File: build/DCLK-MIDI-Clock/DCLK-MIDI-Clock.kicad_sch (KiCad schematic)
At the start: 24 parts, among them J1 MIDI OUT, J2 Jack-DC, J3 MIDI OUT, SW1 CH1, SW2 CH2, SW3 SETTINGS, SW4 RotaryEncoder_Switch_MP

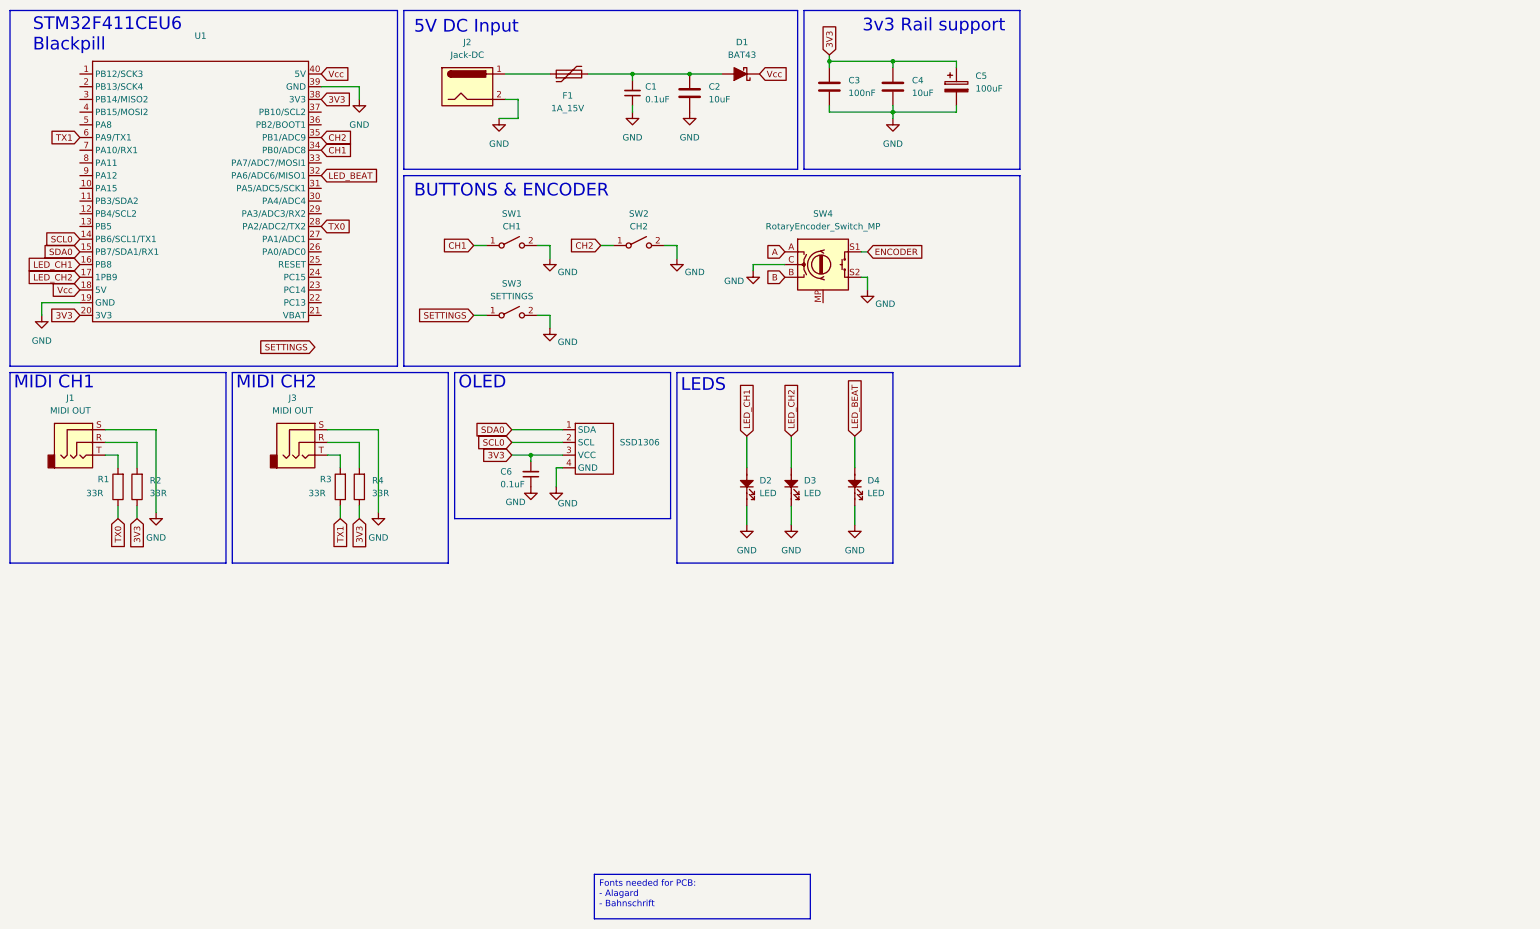
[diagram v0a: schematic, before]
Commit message: pcb rev2
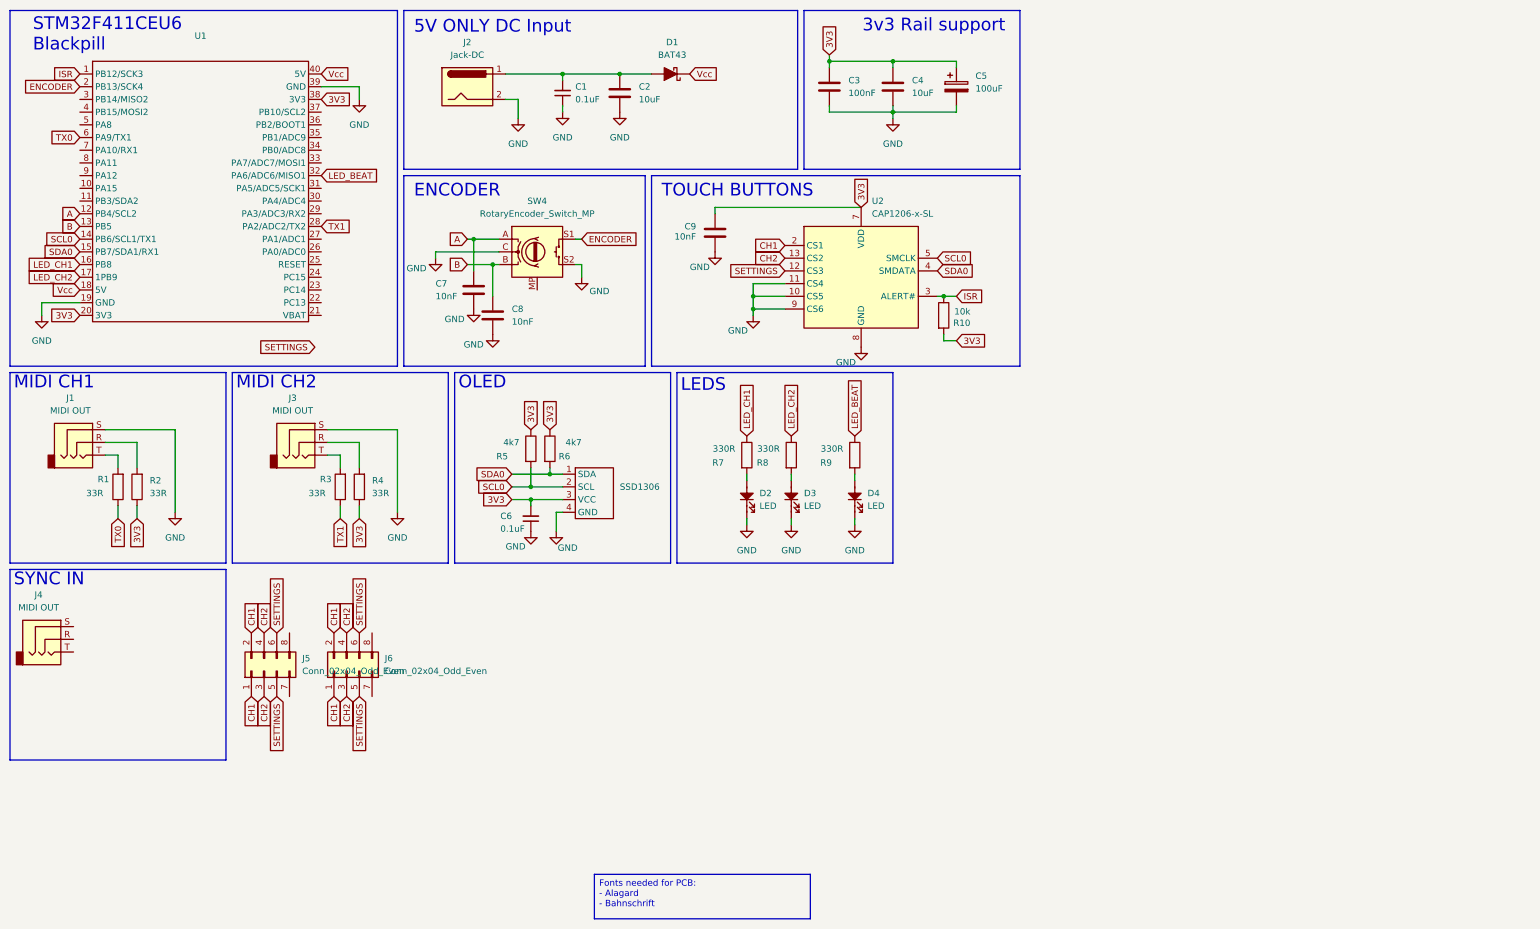
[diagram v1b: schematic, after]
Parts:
- removed F1: 1A_15V, Fuse:Fuse_1812_4532Metric, symbol PCM_4ms_Regulator:Polyfuse_3A_15V
- removed SW1: CH1, Button_Switch_Keyboard:SW_Cherry_MX_1.00u_PCB, symbol Switch:SW_SPST
- removed SW2: CH2, Button_Switch_Keyboard:SW_Cherry_MX_1.00u_PCB, symbol Switch:SW_SPST
- removed SW3: SETTINGS, Button_Switch_Keyboard:SW_Cherry_MX_1.00u_PCB, symbol Switch:SW_SPST
- added C7, C8, C9: 10nF, Capacitor_SMD:C_1206_3216Metric_Pad1.33x1.80mm_HandSolder, symbol Device:C
- added J4: MIDI OUT, audioConnectors_Edit:Jack_3.5mm_CUI_SJ1-3525N_Horizontal_edit, symbol Connector_Audio:AudioJack3
- added J5: Conn_02x04_Odd_Even, Connector_PinSocket_2.54mm:PinSocket_2x04_P2.54mm_Vertical, symbol Connector_Generic:Conn_02x04_Odd_Even
- added J6: Conn_02x04_Odd_Even, Connector_PinHeader_2.54mm:PinHeader_2x04_P2.54mm_Vertical_SMD, symbol Connector_Generic:Conn_02x04_Odd_Even
- added R10: 10k, PCM_4ms_Resistor:R_0603, symbol PCM_4ms_Resistor:10k_0402
- added R5, R6: 4k7, PCM_4ms_Resistor:R_0603, symbol PCM_4ms_Resistor:10k_0402
- added R7, R8, R9: 330R, PCM_4ms_Resistor:R_0603, symbol PCM_4ms_Resistor:10k_0402
- added U2: CAP1206-x-SL, Package_SO:SOIC-14_3.9x8.7mm_P1.27mm, symbol Sensor_Touch:CAP1206-x-SL
- SSD1306: footprint SSD1306_footprint:SSD1306_OLED_Module -> SSD1306:SSD1306-128x32
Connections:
- net 3V3: now also C9.2, R10.2, R5.1, R6.1, U2.7 (VDD)
- net A: now also U1.12 (PB4/SCL2), C7.1
- net B: now also U1.13 (PB5), C8.1
- net CH1: now also J5.1 (Pin_1), J5.2 (Pin_2), J6.1 (Pin_1), J6.2 (Pin_2), U2.2 (CS1); no longer U1.34 (PB0/ADC8)
- net CH2: now also J5.3 (Pin_3), J5.4 (Pin_4), J6.3 (Pin_3), J6.4 (Pin_4), U2.13 (CS2); no longer U1.35 (PB1/ADC9)
- net ENCODER: now also U1.2 (PB13/SCK4)
- net GND: now also C7.2, C8.2, C9.1, U2.10 (CS5), U2.11 (CS4), U2.8 (GND), U2.9 (CS6)
- net LED_BEAT: now also R9.1; no longer D4.2
- net LED_CH1: now also R7.1; no longer D2.2
- net LED_CH2: now also R8.1; no longer D3.2
- net SCL0: now also R5.2, U2.5 (SMCLK)
- net SDA0: now also R6.2, U2.4 (SMDATA)
- net SETTINGS: now also J5.5 (Pin_5), J5.6 (Pin_6), J6.5 (Pin_5), J6.6 (Pin_6), U2.12 (CS3)
- net TX0: now also U1.6 (PA9/TX1); no longer U1.28 (PA2/ADC2/TX2)
- net TX1: now also U1.28 (PA2/ADC2/TX2); no longer U1.6 (PA9/TX1)
- net ISR: now reaches U1.1 (PB12/SCK3)
- net ISR: now also R10.1, U2.3 (ALERT#)
- net at C1.2, C2.1, D1.2 (A): now also J2.1
- new net: D3.2, R8.2
- new net: D4.2, R9.2
- new net: D2.2, R7.2
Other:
- note added: "5V ONLY DC Input"
- note added: "ENCODER"
- note added: "SYNC IN"
- note added: "TOUCH BUTTONS"
- note removed: "5V DC Input"
- note removed: "BUTTONS & ENCODER"
- moved on the sheet: C1, C2, C6, D1, D2, D3, D4, SSD1306, SW4

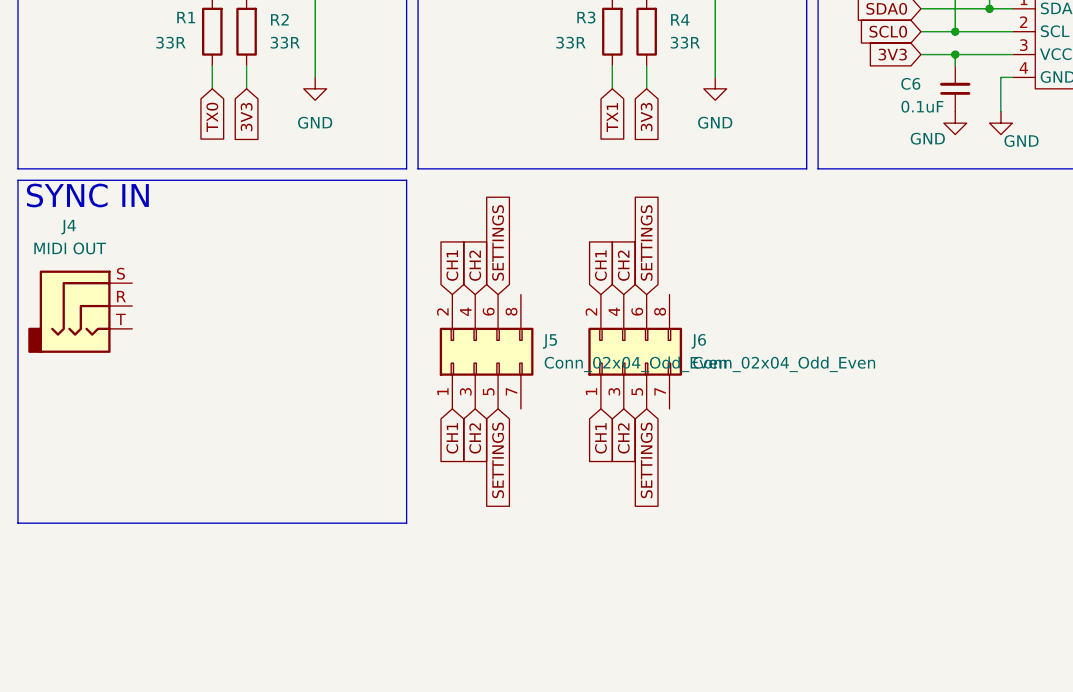
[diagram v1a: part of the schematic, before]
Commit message: pcb rev2
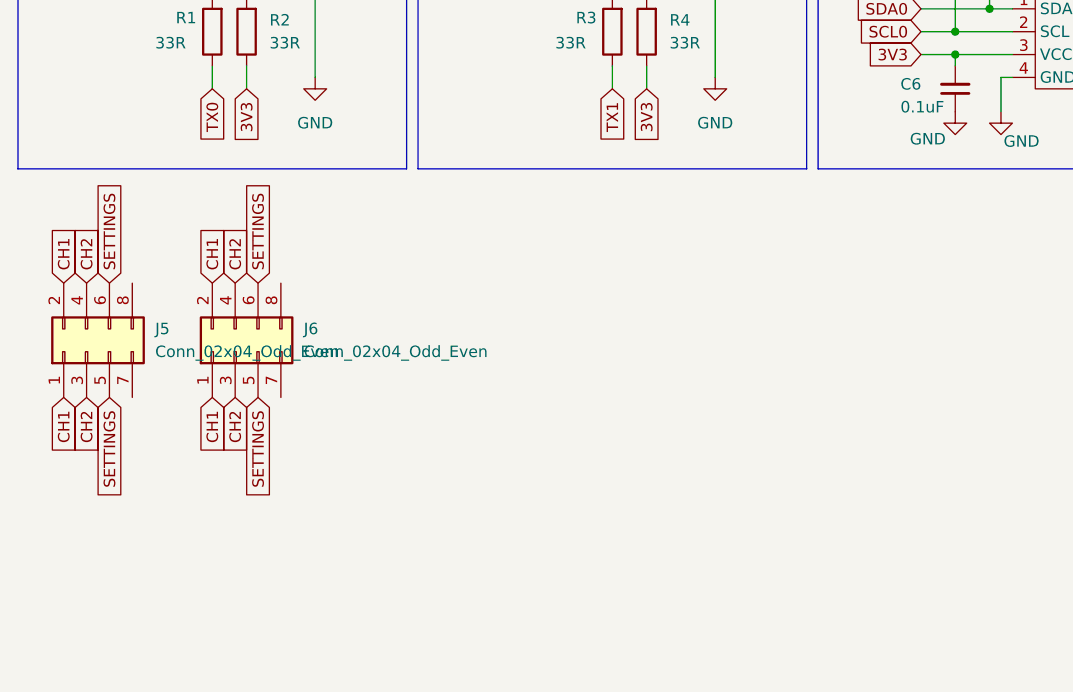
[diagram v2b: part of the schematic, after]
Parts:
- removed J4: MIDI OUT, audioConnectors_Edit:Jack_3.5mm_CUI_SJ1-3525N_Horizontal_edit, symbol Connector_Audio:AudioJack3
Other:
- note removed: "SYNC IN"
- moved on the sheet: J5, J6
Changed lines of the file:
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@@
 	)
 	(rectangle
-		(start 13.97 125.73)
-		(end 57.15 163.83)
-		(stroke
-			(width 0)
-			(type default)
-		)
-		(fill
-			(type none)
-		)
-	)
-	(rectangle
 		(start 102.87 86.36)
 		(end 146.05 124.46)
@@
 		)
 	)
-	(text "SYNC IN"
-		(exclude_from_sim no)
-		(at 14.732 127.762 0)
-		(effects
-			(font
-				(face "Alagard")
-				(size 2.54 2.54)
-			)
-			(justify left)
-		)
-	)
 	(text "MIDI CH2\n"
 		(exclude_from_sim no)
@@
 	(global_label "SETTINGS"
 		(shape input)
-		(at 67.31 151.13 270)
+		(at 24.13 149.86 270)
 		(fields_autoplaced yes)
 		(effects
@@
 		)
 		(property "Intersheetrefs" "${INTERSHEET_REFS}"
-			(at 67.31 162.8237 90)
+			(at 24.13 161.5537 90)
 			(effects
 				(font
@@
 	(global_label "SETTINGS"
 		(shape input)
-		(at 83.82 151.13 270)
+		(at 40.64 149.86 270)
 		(fields_autoplaced yes)
 		(effects
@@
 		)
 		(property "Intersheetrefs" "${INTERSHEET_REFS}"
-			(at 83.82 162.8237 90)
+			(at 40.64 161.5537 90)
 			(effects
 				(font
@@
 	(global_label "CH2"
 		(shape input)
-		(at 81.28 138.43 90)
+		(at 38.1 137.16 90)
 		(fields_autoplaced yes)
 		(effects
@@
 		)
 		(property "Intersheetrefs" "${INTERSHEET_REFS}"
-			(at 81.28 131.6348 90)
+			(at 38.1 130.3648 90)
 			(effects
 				(font
@@
 	(global_label "CH2"
 		(shape input)
-		(at 64.77 151.13 270)
+		(at 21.59 149.86 270)
 		(fields_autoplaced yes)
 		(effects
@@
 		)
 		(property "Intersheetrefs" "${INTERSHEET_REFS}"
-			(at 64.77 157.9252 90)
+			(at 21.59 156.6552 90)
 			(effects
 				(font
@@
 	(global_label "CH2"
 		(shape input)
-		(at 81.28 151.13 270)
+		(at 38.1 149.86 270)
 		(fields_autoplaced yes)
 		(effects
@@
 		)
 		(property "Intersheetrefs" "${INTERSHEET_REFS}"
-			(at 81.28 157.9252 90)
+			(at 38.1 156.6552 90)
 			(effects
 				(font
@@
 	(global_label "CH1"
 		(shape input)
-		(at 62.23 151.13 270)
+		(at 19.05 149.86 270)
 		(fields_autoplaced yes)
 		(effects
@@
 		)
 		(property "Intersheetrefs" "${INTERSHEET_REFS}"
-			(at 62.23 157.9252 90)
+			(at 19.05 156.6552 90)
 			(effects
 				(font
@@
 	(global_label "SETTINGS"
 		(shape input)
-		(at 67.31 138.43 90)
+		(at 24.13 137.16 90)
 		(fields_autoplaced yes)
 		(effects
@@
 		)
 		(property "Intersheetrefs" "${INTERSHEET_REFS}"
-			(at 67.31 126.7363 90)
+			(at 24.13 125.4663 90)
 			(effects
 				(font
@@
 	(global_label "CH1"
 		(shape input)
-		(at 78.74 138.43 90)
+		(at 35.56 137.16 90)
 		(fields_autoplaced yes)
 		(effects
@@
 		)
 		(property "Intersheetrefs" "${INTERSHEET_REFS}"
-			(at 78.74 131.6348 90)
+			(at 35.56 130.3648 90)
 			(effects
 				(font
@@
 	(global_label "CH1"
 		(shape input)
-		(at 62.23 138.43 90)
+		(at 19.05 137.16 90)
 		(fields_autoplaced yes)
 		(effects
@@
 		)
 		(property "Intersheetrefs" "${INTERSHEET_REFS}"
-			(at 62.23 131.6348 90)
+			(at 19.05 130.3648 90)
 			(effects
 				(font
@@
 	(global_label "CH1"
 		(shape input)
-		(at 78.74 151.13 270)
+		(at 35.56 149.86 270)
 		(fields_autoplaced yes)
 		(effects
@@
 		)
 		(property "Intersheetrefs" "${INTERSHEET_REFS}"
-			(at 78.74 157.9252 90)
+			(at 35.56 156.6552 90)
 			(effects
 				(font
@@
 	(global_label "SETTINGS"
 		(shape input)
-		(at 83.82 138.43 90)
+		(at 40.64 137.16 90)
 		(fields_autoplaced yes)
 		(effects
@@
 		)
 		(property "Intersheetrefs" "${INTERSHEET_REFS}"
-			(at 83.82 126.7363 90)
+			(at 40.64 125.4663 90)
 			(effects
 				(font
@@
 	(global_label "CH2"
 		(shape input)
-		(at 64.77 138.43 90)
+		(at 21.59 137.16 90)
 		(fields_autoplaced yes)
 		(effects
@@
 		)
 		(property "Intersheetrefs" "${INTERSHEET_REFS}"
-			(at 64.77 131.6348 90)
+			(at 21.59 130.3648 90)
 			(effects
 				(font
@@
 	(symbol
 		(lib_id "Connector_Generic:Conn_02x04_Odd_Even")
-		(at 64.77 146.05 90)
+		(at 21.59 144.78 90)
 		(unit 1)
 		(exclude_from_sim no)
@@
 		(fields_autoplaced yes)
 		(property "Reference" "J5"
-			(at 72.39 143.5099 90)
+			(at 29.21 142.2399 90)
 			(effects
 				(font
@@
 		)
 		(property "Value" "Conn_02x04_Odd_Even"
-			(at 72.39 146.0499 90)
+			(at 29.21 144.7799 90)
 			(effects
 				(font
@@
 		)
 		(property "Footprint" "Connector_PinSocket_2.54mm:PinSocket_2x04_P2.54mm_Vertical"
-			(at 64.77 146.05 0)
+			(at 21.59 144.78 0)
 			(effects
 				(font
@@
 		)
 		(property "Datasheet" "~"
-			(at 64.77 146.05 0)
+			(at 21.59 144.78 0)
 			(effects
 				(font
@@
 		)
 		(property "Description" "Generic connector, double row, 02x04, odd/even pin numbering scheme (row 1 odd numbers, row 2 even numbers), script generated (kicad-library-utils/schlib/autogen/connector/)"
-			(at 64.77 146.05 0)
+			(at 21.59 144.78 0)
 			(effects
 				(font
@@
 	)
 	(symbol
-		(lib_id "Connector_Audio:AudioJack3")
-		(at 21.59 139.7 0)
-		(unit 1)
-		(exclude_from_sim no)
-		(in_bom yes)
-		(on_board yes)
-		(dnp no)
-		(fields_autoplaced yes)
-		(property "Reference" "J4"
-			(at 19.685 130.81 0)
-			(effects
-				(font
-					(size 1.27 1.27)
-				)
-			)
-		)
-		(property "Value" "MIDI OUT"
-			(at 19.685 133.35 0)
-			(effects
-				(font
-					(size 1.27 1.27)
-				)
-			)
-		)
-		(property "Footprint" "audioConnectors_Edit:Jack_3.5mm_CUI_SJ1-3525N_Horizontal_edit"
-			(at 21.59 139.7 0)
-			(effects
-				(font
-					(size 1.27 1.27)
-				)
-				(hide yes)
-			)
-		)
-		(property "Datasheet" "~"
-			(at 21.59 139.7 0)
-			(effects
-				(font
-					(size 1.27 1.27)
-				)
-				(hide yes)
-			)
-		)
-		(property "Description" "Audio Jack, 3 Poles (Stereo / TRS)"
-			(at 21.59 139.7 0)
-			(effects
-				(font
-					(size 1.27 1.27)
-				)
-				(hide yes)
-			)
-		)
-		(pin "S"
-		)
-		(pin "T"
-		)
-		(pin "R"
-		)
-		(instances
-			(project "DCLK-MIDI-Clock"
-				(path "/42d00d8e-48e3-47e6-b456-ac5bd2d9bc78"
-					(reference "J4")
-					(unit 1)
-				)
-			)
-		)
-	)
-	(symbol
 		(lib_id "power:GND")
 		(at 190.5 35.56 0)
@@
 	(symbol
 		(lib_id "Connector_Generic:Conn_02x04_Odd_Even")
-		(at 81.28 146.05 90)
+		(at 38.1 144.78 90)
 		(unit 1)
 		(exclude_from_sim no)
@@
 		(fields_autoplaced yes)
 		(property "Reference" "J6"
-			(at 88.9 143.5099 90)
+			(at 45.72 142.2399 90)
 			(effects
 				(font
@@
 		)
 		(property "Value" "Conn_02x04_Odd_Even"
-			(at 88.9 146.0499 90)
+			(at 45.72 144.7799 90)
 			(effects
 				(font
@@
 		)
 		(property "Footprint" "Connector_PinHeader_2.54mm:PinHeader_2x04_P2.54mm_Vertical_SMD"
-			(at 81.28 146.05 0)
+			(at 38.1 144.78 0)
 			(effects
 				(font
@@
 		)
 		(property "Datasheet" "~"
-			(at 81.28 146.05 0)
+			(at 38.1 144.78 0)
 			(effects
 				(font
@@
 		)
 		(property "Description" "Generic connector, double row, 02x04, odd/even pin numbering scheme (row 1 odd numbers, row 2 even numbers), script generated (kicad-library-utils/schlib/autogen/connector/)"
-			(at 81.28 146.05 0)
+			(at 38.1 144.78 0)
 			(effects
 				(font
